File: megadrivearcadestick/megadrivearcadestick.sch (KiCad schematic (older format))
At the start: 26 parts

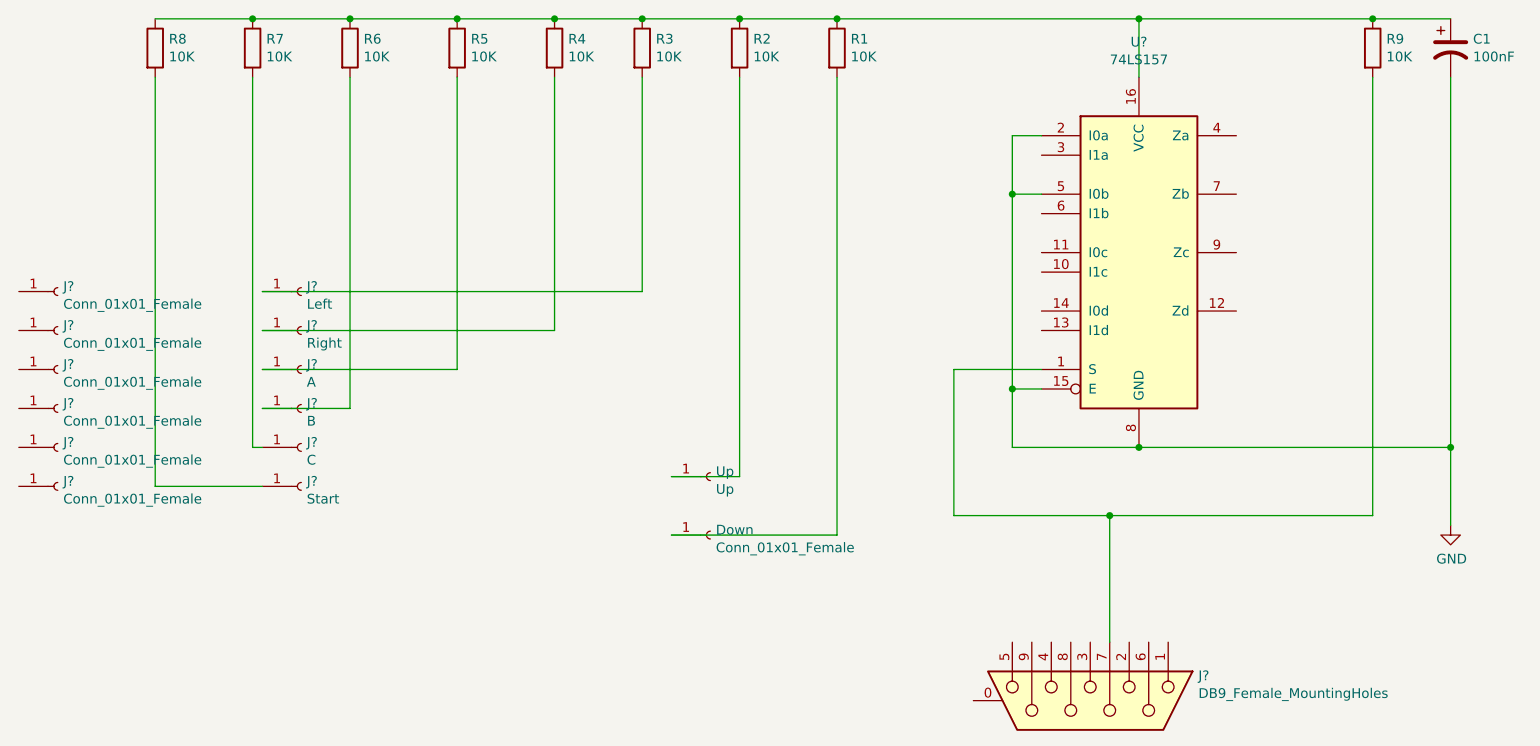
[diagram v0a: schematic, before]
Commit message: Better schematics
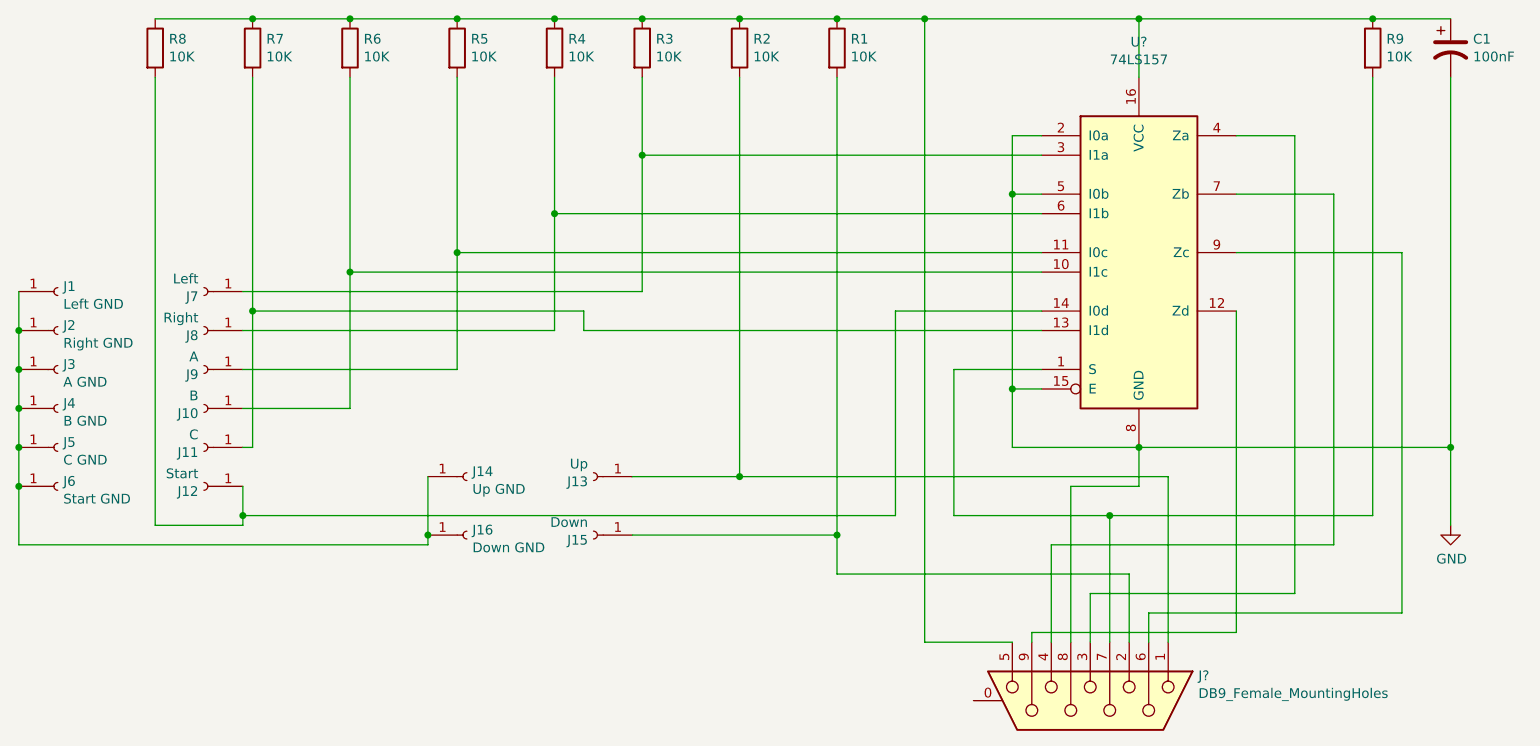
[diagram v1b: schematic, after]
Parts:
- added J14: Up GND, symbol Connector:Conn_01x01_Female
- added J16: Down GND, symbol Connector:Conn_01x01_Female
- J1: renamed from J?; value Conn_01x01_Female -> Left GND
- J15: renamed from Down; value Conn_01x01_Female -> Down
- J2: renamed from J?; value Conn_01x01_Female -> Right GND
- J3: renamed from J?; value Conn_01x01_Female -> A GND
- J4: renamed from J?; value Conn_01x01_Female -> B GND
- J5: renamed from J?; value Conn_01x01_Female -> C GND
- J6: renamed from J?; value Conn_01x01_Female -> Start GND
- gave numbers to parts that had none: 6
- renumbered Up to J13
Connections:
- net GND: now also J?.8
- net at C1.1, R1.1, R2.1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: now also J?.5
- net at J12.1 (Pin_1), R8.2: now also U?.14 (I0d)
- net at J11.1 (Pin_1), R7.2: now also U?.13 (I1d)
- net at J10.1 (Pin_1), R6.2: now also U?.10 (I1c)
- net at J9.1 (Pin_1), R5.2: now also U?.11 (I0c)
- net at J8.1 (Pin_1), R4.2: now also U?.6 (I1b)
- net at J7.1 (Pin_1), R3.2: now also U?.3 (I1a)
- net at J13.1 (Pin_1), R2.2: now also J?.1
- net at J15.1 (Pin_1), R1.2: now also J?.2
- net at U?.12 (Zd): now also J?.9
- net at U?.4 (Za): now also J?.3
- net at U?.7 (Zb): now also J?.4
- net at U?.9 (Zc): now also J?.6
- net at J1.1 (Pin_1): now also J2.1 (Pin_1), J3.1 (Pin_1), J4.1 (Pin_1), J5.1 (Pin_1), J6.1 (Pin_1), J14.1 (Pin_1), J16.1 (Pin_1)
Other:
- moved on the sheet: J10, J11, J12, J13, J15, J7, J8, J9
